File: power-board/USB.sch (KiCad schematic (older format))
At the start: 6 parts, among them J1101 USB_OTG, U1101 TPD2E001IDRLRQ1

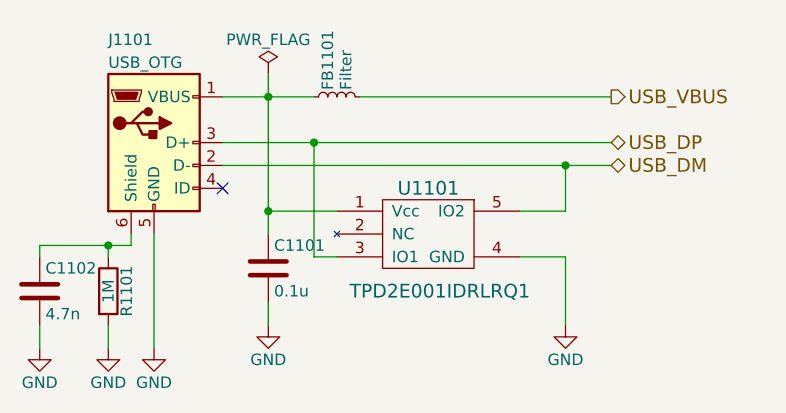
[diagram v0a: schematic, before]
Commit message: routed board
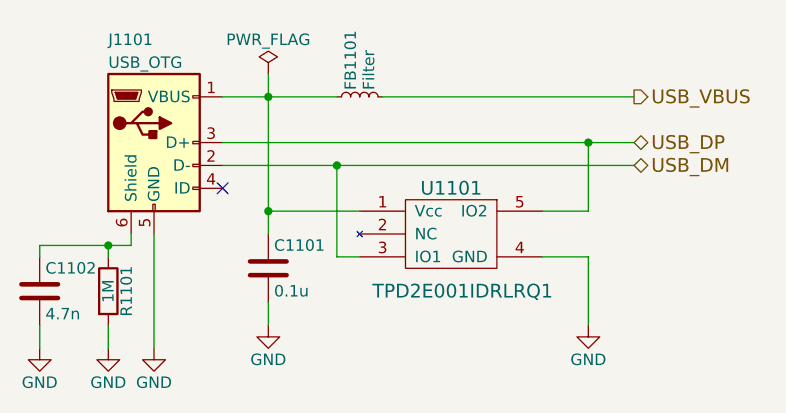
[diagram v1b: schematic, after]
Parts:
- C1101: footprint (none) -> Capacitors_SMD:C_0603; MFG (none) -> Murata Electronics; MPN (none) -> GRM188R71H104KA93D
- C1102: footprint (none) -> Capacitors_SMD:C_0603; MFG (none) -> Samsung; MPN (none) -> CL10B472KB8NNNC
- FB1101: footprint (none) -> Resistors_SMD:R_0805; MFG (none) -> TDK; MPN (none) -> MPZ2012S102AT000
- J1101: footprint (none) -> Connectors:USB_Micro-B_10103594-0001LF; MFG (none) -> Amphenol FCI; MPN (none) -> 10103594-0001LF
- R1101: footprint (none) -> Resistors_SMD:R_0603; MFG (none) -> Yageo; MPN (none) -> RC0603JR-071ML
- U1101: footprint SOT553 -> TO_SOT_Packages_SMD:SOT-553
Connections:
- net USB_DM: now also U1101.3 (IO1); no longer U1101.5 (IO2)
- net USB_DP: now also U1101.5 (IO2); no longer U1101.3 (IO1)
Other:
- moved on the sheet: FB1101, U1101
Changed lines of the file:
@@
 $Descr A4 11693 8268
 encoding utf-8
-Sheet 11 11
+Sheet 11 12
 Title ""
 Date ""
@@
 Comment4 ""
 $EndDescr
-Text HLabel 6900 3600 2    60   BiDi ~ 0
+Text HLabel 7000 3600 2    60   BiDi ~ 0
 USB_DM
-Text HLabel 6900 3500 2    60   BiDi ~ 0
+Text HLabel 7000 3500 2    60   BiDi ~ 0
 USB_DP
 $Comp
@@
 F 0 "J1101" H 4700 3950 50  0000 L CNN
 F 1 "USB_OTG" H 4700 3850 50  0000 L CNN
-F 2 "" H 5050 3450 50  0001 C CNN
+F 2 "Connectors:USB_Micro-B_10103594-0001LF" H 5050 3450 50  0001 C CNN
 F 3 "" H 5050 3450 50  0001 C CNN
+F 4 "Amphenol FCI" H 4900 3500 60  0001 C CNN "MFG"
+F 5 "10103594-0001LF" H 4900 3500 60  0001 C CNN "MPN"
 	1    4900 3500
 	1    0    0    -1
@@
 L TPD2E001IDRLRQ1 U1101
 U 1 1 593D62EE
-P 6100 3950
-F 0 "U1101" H 6100 4200 60  0000 C CNN
-F 1 "TPD2E001IDRLRQ1" H 6150 3750 60  0000 C CNN
-F 2 "SOT553" H 6100 3950 60  0001 C CNN
-F 3 "" H 6100 3950 60  0000 C CNN
-F 4 "Texas Instruments" H 6200 4300 60  0001 C CNN "MFG"
-F 5 "TPD2E001IDRLRQ1" H 6300 4400 60  0001 C CNN "MPN"
-	1    6100 3950
-	1    0    0    -1
-$EndComp
-Wire Wire Line
-	5200 3500 6900 3500
-Wire Wire Line
-	5200 3600 6900 3600
-Wire Wire Line
-	5200 3300 5600 3300
-Wire Wire Line
-	5700 3800 5400 3800
+P 6200 3950
+F 0 "U1101" H 6200 4200 60  0000 C CNN
+F 1 "TPD2E001IDRLRQ1" H 6250 3750 60  0000 C CNN
+F 2 "TO_SOT_Packages_SMD:SOT-553" H 6200 3950 60  0001 C CNN
+F 3 "" H 6200 3950 60  0000 C CNN
+F 4 "Texas Instruments" H 6300 4300 60  0001 C CNN "MFG"
+F 5 "TPD2E001IDRLRQ1" H 6400 4400 60  0001 C CNN "MPN"
+	1    6200 3950
+	1    0    0    -1
+$EndComp
+Wire Wire Line
+	5200 3500 7000 3500
+Wire Wire Line
+	5200 3600 7000 3600
+Wire Wire Line
+	5200 3300 5700 3300
+Wire Wire Line
+	5400 3800 5800 3800
 Wire Wire Line
 	5400 3200 5400 3900
 Connection ~ 5400 3300
 Wire Wire Line
-	5700 4000 5600 4000
-Wire Wire Line
-	5600 4000 5600 3500
-Connection ~ 5600 3500
-Wire Wire Line
-	6500 3800 6700 3800
-Wire Wire Line
-	6700 3800 6700 3600
-Connection ~ 6700 3600
-$Comp
-L C C1101
-U 1 1 593D63F8
-P 5400 4050
-F 0 "C1101" H 5425 4150 50  0000 L CNN
-F 1 "0.1u" H 5425 3950 50  0000 L CNN
-F 2 "" H 5438 3900 50  0001 C CNN
-F 3 "" H 5400 4050 50  0001 C CNN
-	1    5400 4050
-	1    0    0    -1
-$EndComp
+	5800 4000 5700 4000
+Wire Wire Line
+	6600 3800 6800 3800
 Connection ~ 5400 3800
 Wire Wire Line
 	5400 4300 5400 4200
 $Comp
-L GND #PWR054
+L GND #PWR040
 U 1 1 593D649D
 P 5400 4300
-F 0 "#PWR054" H 5400 4050 50  0001 C CNN
+F 0 "#PWR040" H 5400 4050 50  0001 C CNN
 F 1 "GND" H 5400 4150 50  0000 C CNN
 F 2 "" H 5400 4300 50  0001 C CNN
@@
 $EndComp
 $Comp
-L GND #PWR055
+L GND #PWR041
 U 1 1 593D64C8
-P 6700 4300
-F 0 "#PWR055" H 6700 4050 50  0001 C CNN
-F 1 "GND" H 6700 4150 50  0000 C CNN
-F 2 "" H 6700 4300 50  0001 C CNN
-F 3 "" H 6700 4300 50  0001 C CNN
-	1    6700 4300
-	1    0    0    -1
-$EndComp
-Wire Wire Line
-	6500 4000 6700 4000
-Wire Wire Line
-	6700 4000 6700 4300
-$Comp
-L GND #PWR056
+P 6800 4300
+F 0 "#PWR041" H 6800 4050 50  0001 C CNN
+F 1 "GND" H 6800 4150 50  0000 C CNN
+F 2 "" H 6800 4300 50  0001 C CNN
+F 3 "" H 6800 4300 50  0001 C CNN
+	1    6800 4300
+	1    0    0    -1
+$EndComp
+Wire Wire Line
+	6600 4000 6800 4000
+Wire Wire Line
+	6800 4000 6800 4300
+$Comp
+L GND #PWR042
 U 1 1 593D64F9
 P 4900 4400
-F 0 "#PWR056" H 4900 4150 50  0001 C CNN
+F 0 "#PWR042" H 4900 4150 50  0001 C CNN
 F 1 "GND" H 4900 4250 50  0000 C CNN
 F 2 "" H 4900 4400 50  0001 C CNN
@@
 Wire Wire Line
 	4900 3900 4900 4400
-$Comp
-L C C1102
-U 1 1 593D6523
-P 4400 4150
-F 0 "C1102" H 4425 4250 50  0000 L CNN
-F 1 "4.7n" H 4425 4050 50  0000 L CNN
-F 2 "" H 4438 4000 50  0001 C CNN
-F 3 "" H 4400 4150 50  0001 C CNN
-	1    4400 4150
-	1    0    0    -1
-$EndComp
 $Comp
 L R R1101
@@
 F 0 "R1101" V 4780 4150 50  0000 C CNN
 F 1 "1M" V 4700 4150 50  0000 C CNN
-F 2 "" V 4630 4150 50  0001 C CNN
+F 2 "Resistors_SMD:R_0603" V 4630 4150 50  0001 C CNN
 F 3 "" H 4700 4150 50  0001 C CNN
+F 4 "Yageo" V 4700 4150 60  0001 C CNN "MFG"
+F 5 "RC0603JR-071ML" V 4700 4150 60  0001 C CNN "MPN"
 	1    4700 4150
 	1    0    0    -1
 $EndComp
 $Comp
-L GND #PWR057
+L GND #PWR043
 U 1 1 593D65FF
 P 4700 4400
-F 0 "#PWR057" H 4700 4150 50  0001 C CNN
+F 0 "#PWR043" H 4700 4150 50  0001 C CNN
 F 1 "GND" H 4700 4250 50  0000 C CNN
 F 2 "" H 4700 4400 50  0001 C CNN
@@
 	4700 4400 4700 4300
 $Comp
-L GND #PWR058
+L GND #PWR044
 U 1 1 593D6635
 P 4400 4400
-F 0 "#PWR058" H 4400 4150 50  0001 C CNN
+F 0 "#PWR044" H 4400 4150 50  0001 C CNN
 F 1 "GND" H 4400 4250 50  0000 C CNN
 F 2 "" H 4400 4400 50  0001 C CNN
@@
 	4700 4000 4700 3950
 Connection ~ 4700 3950
-Text HLabel 6900 3300 2    60   Output ~ 0
+Text HLabel 7000 3300 2    60   Output ~ 0
 USB_VBUS
 $Comp
 L L_Small FB1101
 U 1 1 593D6AFC
-P 5700 3300
-F 0 "FB1101" H 5730 3340 50  0000 L CNN
-F 1 "Filter" H 5730 3260 50  0000 L CNN
-F 2 "" H 5700 3300 50  0001 C CNN
-F 3 "" H 5700 3300 50  0001 C CNN
-	1    5700 3300
+P 5800 3300
+F 0 "FB1101" H 5830 3340 50  0000 L CNN
+F 1 "Filter" H 5830 3260 50  0000 L CNN
+F 2 "Resistors_SMD:R_0805" H 5800 3300 50  0001 C CNN
+F 3 "" H 5800 3300 50  0001 C CNN
+F 4 "TDK" H 5800 3300 60  0001 C CNN "MFG"
+F 5 "MPZ2012S102AT000" H 5800 3300 60  0001 C CNN "MPN"
+	1    5800 3300
 	0    -1   -1   0
 $EndComp
 Wire Wire Line
-	5800 3300 6900 3300
-$Comp
-L PWR_FLAG #FLG059
+	5900 3300 7000 3300
+$Comp
+L PWR_FLAG #FLG045
 U 1 1 593DC797
 P 5400 3200
-F 0 "#FLG059" H 5400 3275 50  0001 C CNN
+F 0 "#FLG045" H 5400 3275 50  0001 C CNN
 F 1 "PWR_FLAG" H 5400 3350 50  0000 C CNN
 F 2 "" H 5400 3200 50  0001 C CNN
@@
 	1    0    0    -1
 $EndComp
+$Comp
+L C C1101
+U 1 1 593E3D68
+P 5400 4050
+F 0 "C1101" H 5425 4150 50  0000 L CNN
+F 1 "0.1u" H 5425 3950 50  0000 L CNN
+F 2 "Capacitors_SMD:C_0603" H 5438 3900 50  0001 C CNN
+F 3 "" H 5400 4050 50  0000 C CNN
+F 4 "Murata Electronics" H 5400 4050 60  0001 C CNN "MFG"
+F 5 "GRM188R71H104KA93D" H 5400 4050 60  0001 C CNN "MPN"
+	1    5400 4050
+	1    0    0    -1
+$EndComp
+$Comp
+L C C1102
+U 1 1 593E44E8
+P 4400 4150
+F 0 "C1102" H 4425 4250 50  0000 L CNN
+F 1 "4.7n" H 4425 4050 50  0000 L CNN
+F 2 "Capacitors_SMD:C_0603" H 4438 4000 50  0001 C CNN
+F 3 "" H 4400 4150 50  0000 C CNN
+F 4 "Samsung" H 4400 4150 60  0001 C CNN "MFG"
+F 5 "CL10B472KB8NNNC" H 4400 4150 60  0001 C CNN "MPN"
+	1    4400 4150
+	1    0    0    -1
+$EndComp
+Wire Wire Line
+	5700 4000 5700 3600
+Connection ~ 5700 3600
+Wire Wire Line
+	6800 3800 6800 3500
+Connection ~ 6800 3500
 $EndSCHEMATC
